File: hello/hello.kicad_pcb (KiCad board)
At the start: 2 copper layers, 12 parts, among them J1 pwm, J2 voltmeter, J3 common, J4 continuous, J5 common, SW1 SW_SPST, U1 Arduino nano, U2 oled i2c, U3 Rotary Encoder

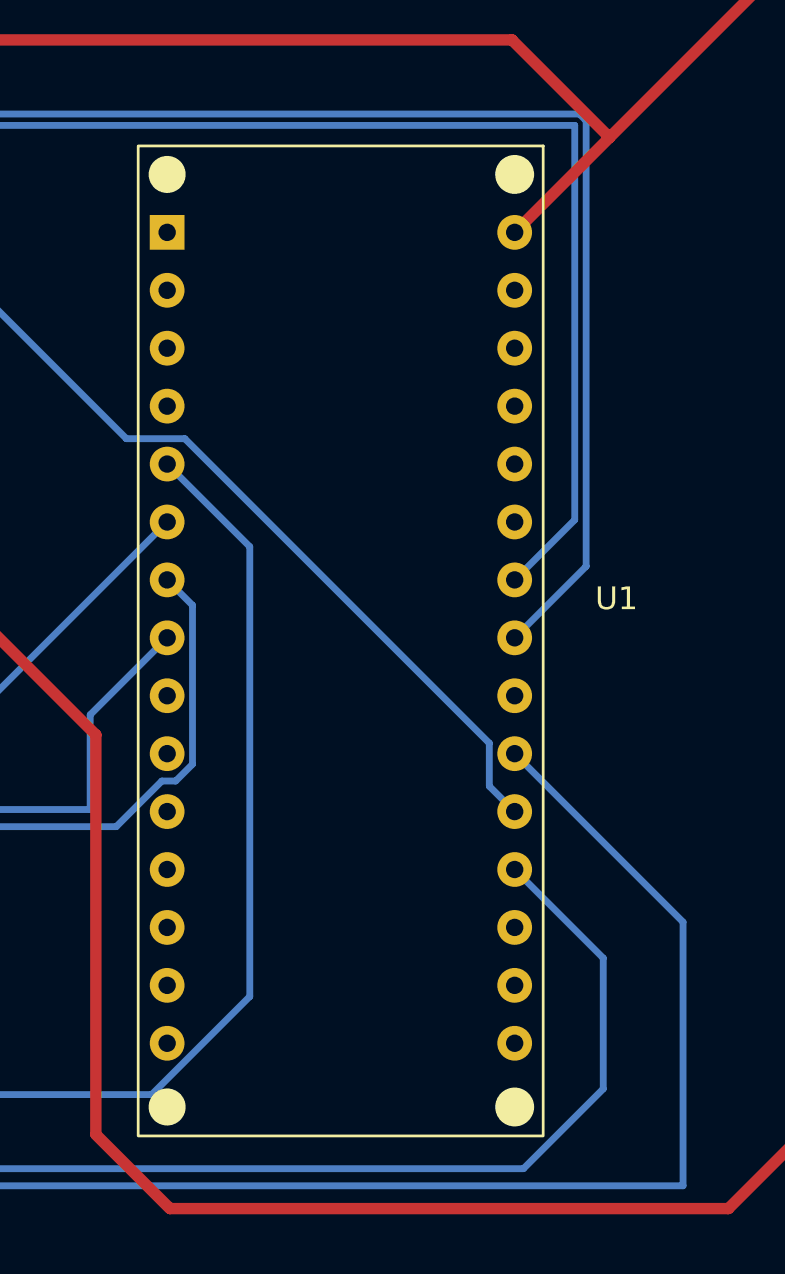
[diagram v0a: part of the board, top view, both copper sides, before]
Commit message: updates to final pcb design
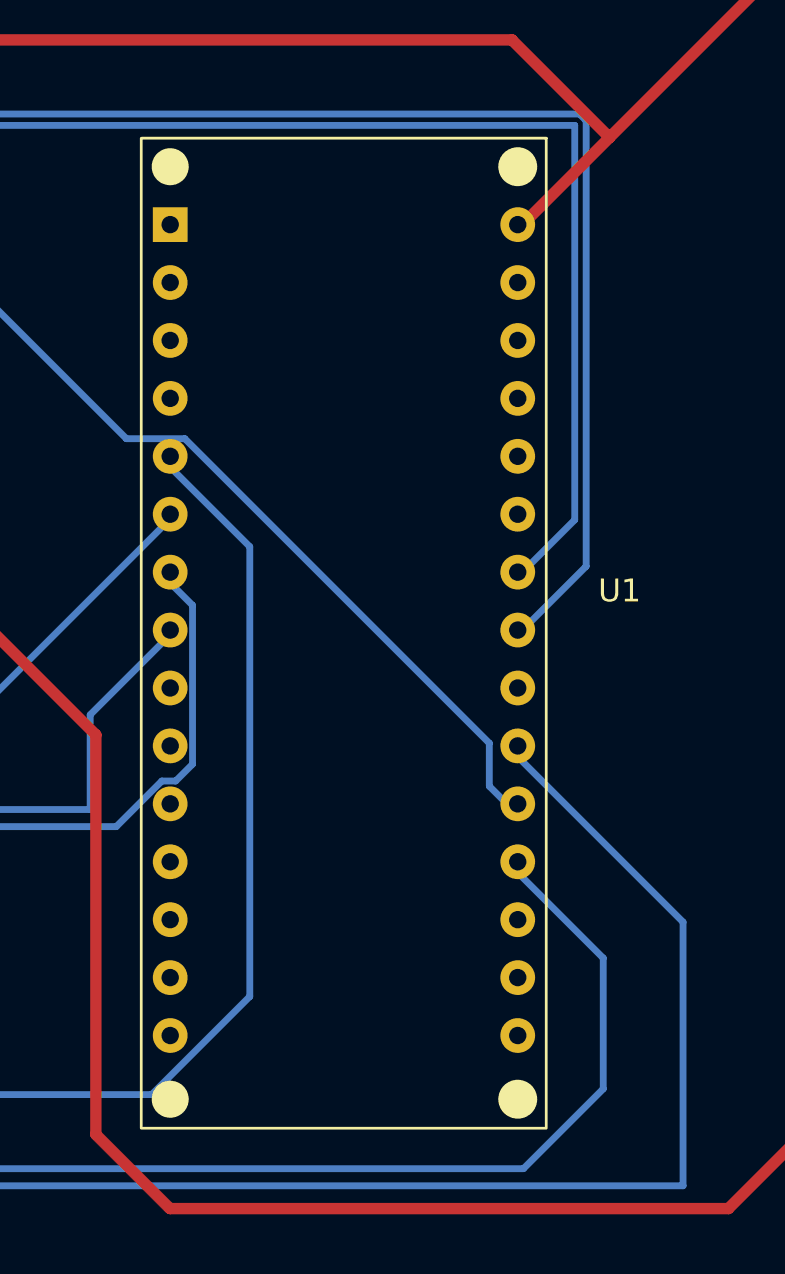
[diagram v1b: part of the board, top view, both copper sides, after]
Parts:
- moved U1 0.37 mm to (142.4, 94.9)
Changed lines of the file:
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@@
 		(tags "Through hole socket strip THT 1x01 1.27mm single row")
 		(property "Reference" "J4"
-			(at 0 -2.135 360)
+			(at 0 -2.135 0)
 			(layer "F.SilkS")
 			(effects
@@
 		)
 		(property "Value" "continuous"
-			(at 0 2.135 360)
+			(at 0 2.135 0)
 			(layer "F.Fab")
 			(effects
@@
 		)
 		(fp_text user "${REFERENCE}"
-			(at 0 0 360)
+			(at 0 0 0)
 			(layer "F.Fab")
 			(effects
@@
 		(tags "Through hole socket strip THT 1x01 1.27mm single row")
 		(property "Reference" "J2"
-			(at 0 -2.135 360)
+			(at 0 -2.135 0)
 			(layer "F.SilkS")
 			(effects
@@
 		)
 		(property "Value" "voltmeter"
-			(at 0 2.135 360)
+			(at 0 2.135 0)
 			(layer "F.Fab")
 			(effects
@@
 		)
 		(fp_text user "${REFERENCE}"
-			(at 0 0 360)
+			(at 0 0 0)
 			(layer "F.Fab")
 			(effects
@@
 		(tags "Through hole socket strip THT 1x04 1.27mm single row")
 		(property "Reference" "U2"
-			(at 0 -3 360)
+			(at 0 -3 0)
 			(layer "F.SilkS")
 			(effects
@@
 		)
 		(fp_text user "${REFERENCE}"
-			(at 0 1.905 360)
+			(at 0 1.905 0)
 			(layer "F.Fab")
 			(effects
@@
 		(tags "Through hole socket strip THT 1x05 1.27mm single row")
 		(property "Reference" "U3"
-			(at 0 -2.69 360)
+			(at 0 -2.69 0)
 			(layer "F.SilkS")
 			(effects
@@
 		)
 		(fp_text user "${REFERENCE}"
-			(at 0 2.54 360)
+			(at 0 2.54 0)
 			(layer "F.Fab")
 			(effects
@@
 		(tags "Through hole socket strip THT 1x01 1.27mm single row")
 		(property "Reference" "J5"
-			(at 0 -2.135 360)
+			(at 0 -2.135 0)
 			(layer "F.SilkS")
 			(effects
@@
 		)
 		(property "Value" "common"
-			(at 0 2.135 360)
+			(at 0 2.135 0)
 			(layer "F.Fab")
 			(effects
@@
 		)
 		(fp_text user "${REFERENCE}"
-			(at 0 0 360)
+			(at 0 0 0)
 			(layer "F.Fab")
 			(effects
@@
 		(tags "Resistor Axial_DIN0204 series Axial Vertical pin pitch 1.9mm 0.167W length 3.6mm diameter 1.6mm")
 		(property "Reference" "R1"
-			(at 0.95 -1.92 360)
+			(at 0.95 -1.92 0)
 			(layer "F.SilkS")
 			(effects
@@
 		)
 		(property "Value" "1k"
-			(at 0.95 1.92 360)
+			(at 0.95 1.92 0)
 			(layer "F.Fab")
 			(effects
@@
 		)
 		(fp_text user "${REFERENCE}"
-			(at 0.95 -1.92 360)
+			(at 0.95 -1.92 0)
 			(layer "F.Fab")
 			(effects
@@
 	(footprint "MCU_arduino_nano:Arduino_nano"
 		(layer "F.Cu")
-		(at 142.25 95.192 -90)
+		(at 142.384 94.852 -90)
 		(property "Reference" "U1"
 			(at 0.0575 -11.8295 0)
@@
 			(pinfunction "VIN")
 			(pintype "input")
+		)
+		(model "C:/Users/arnav/Downloads/Arduino_Nano.STEP"
+			(offset
+				(xyz -20 -9 0)
+			)
+			(scale
+				(xyz 1 1 1)
+			)
+			(rotate
+				(xyz 90 180 180)
+			)
 		)
 	)
@@
 		(tags "Through hole socket strip THT 1x02 1.27mm single row")
 		(property "Reference" "R2"
-			(at -0.27 -2.75 360)
+			(at -0.27 -2.75 0)
 			(layer "F.SilkS")
 			(effects
@@
 		)
 		(fp_text user "${REFERENCE}"
-			(at 0 0.635 360)
+			(at 0 0.635 0)
 			(layer "F.Fab")
 			(effects
@@
 		(tags "Through hole socket strip THT 1x01 1.27mm single row")
 		(property "Reference" "J3"
-			(at 0 -2.135 360)
+			(at 0 -2.135 0)
 			(layer "F.SilkS")
 			(effects
@@
 		)
 		(property "Value" "common"
-			(at 0 2.135 360)
+			(at 0 2.135 0)
 			(layer "F.Fab")
 			(effects
@@
 		)
 		(fp_text user "${REFERENCE}"
-			(at 0 0 360)
+			(at 0 0 0)
 			(layer "F.Fab")
 			(effects
@@
 		(tags "Through hole socket strip THT 1x01 1.27mm single row")
 		(property "Reference" "J1"
-			(at 0 -2.135 360)
+			(at 0 -2.135 0)
 			(layer "F.SilkS")
 			(effects
@@
 		)
 		(property "Value" "pwm"
-			(at 0 2.135 360)
+			(at 0 2.135 0)
 			(layer "F.Fab")
 			(effects
@@
 		)
 		(fp_text user "${REFERENCE}"
-			(at 0 0 360)
-			(layer "F.Fab")
-			(effects
+			(at 0 0 0)
+			(layer "F.Fab")
+			(effects
